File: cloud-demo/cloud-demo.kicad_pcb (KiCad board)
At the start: 2 copper layers, 5 parts, among them J1 Conn_02x02_Counter_Clockwise

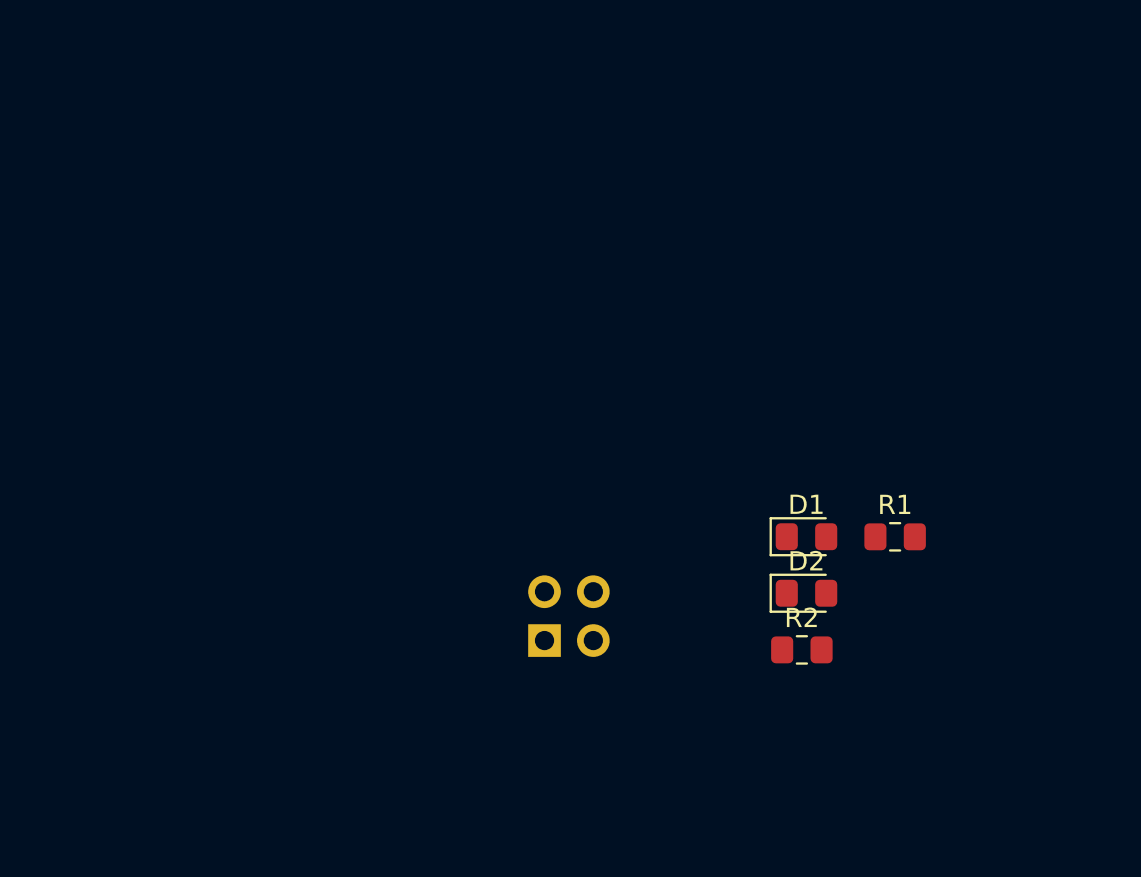
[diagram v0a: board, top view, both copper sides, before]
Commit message: Update demo projects
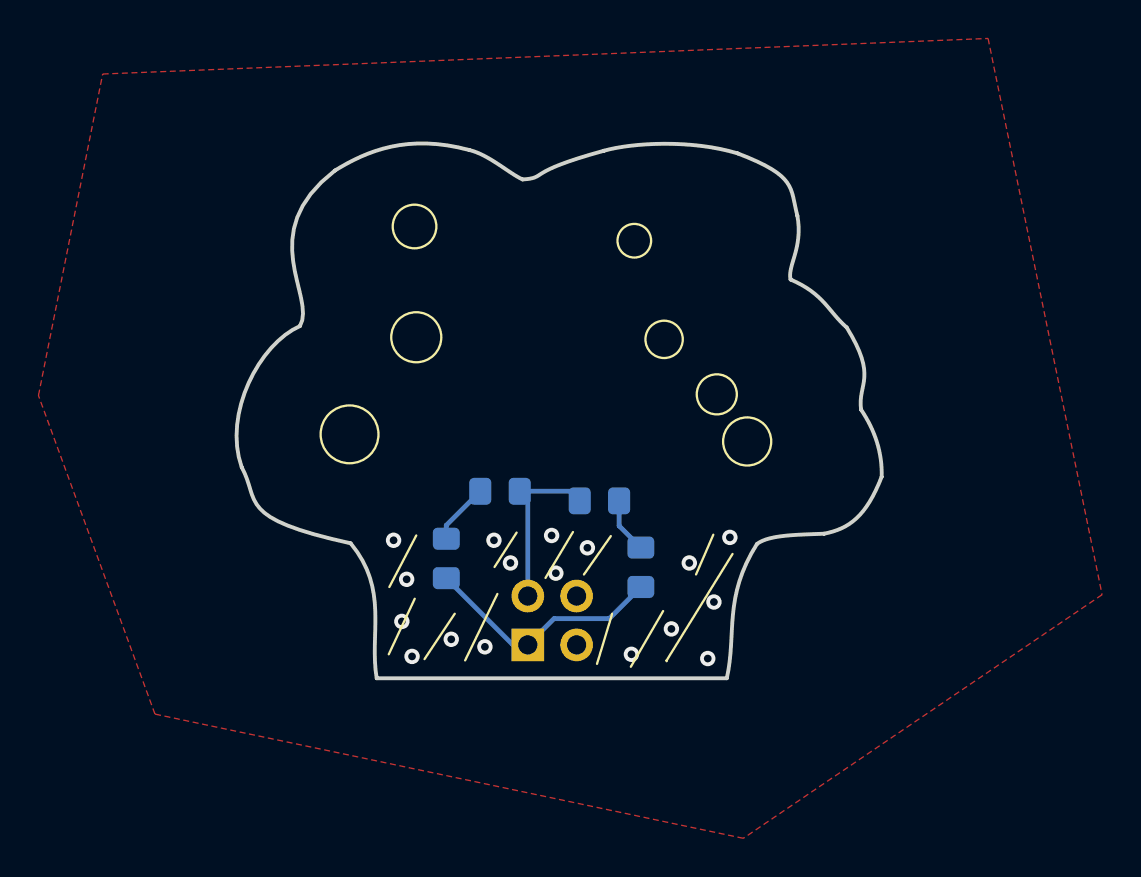
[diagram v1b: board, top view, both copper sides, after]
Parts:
- added G***: LOGO, cloud:bladder, B.Cu at (130.7, 81.9)
- added G***: LOGO, cloud:bladder, B.Cu at (123.2, 81.7)
- added G***: LOGO, cloud:snake, B.Cu at (131.3, 77.7)
- added G***: LOGO, cloud:snake, B.Cu at (132.1, 75.2)
- added G***: LOGO, cloud:cloud, F.Cu at (131.1, 82.0)
- D1, D2, R1, R2: moved to B.Cu
- moved D2 18.8 mm to (125.2, 90.3), turned to 90 degrees
- moved R2 17.7 mm to (128.0, 86.8)
- moved R1 15.5 mm to (133.2, 87.3), turned to 180 degrees
- moved D1 8.76 mm to (135.3, 90.7), turned to 90 degrees
- moved J1 0.90 mm to (129.4, 94.8)
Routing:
- net GND: track 0.00 -> 12.8 mm
- net VCC: track 0.00 -> 8.95 mm
- net Net-(D2-Pad2): track 0.00 -> 3.20 mm
- net Net-(D1-Pad2): track 0.00 -> 2.90 mm
- net (no net): vias 0 -> 17
- added copper zone on F.Cu, net (none)
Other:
- board outline added: 33.6 x 27.8 mm
